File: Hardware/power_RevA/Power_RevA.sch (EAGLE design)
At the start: 11 parts, among them Q401 TIP120

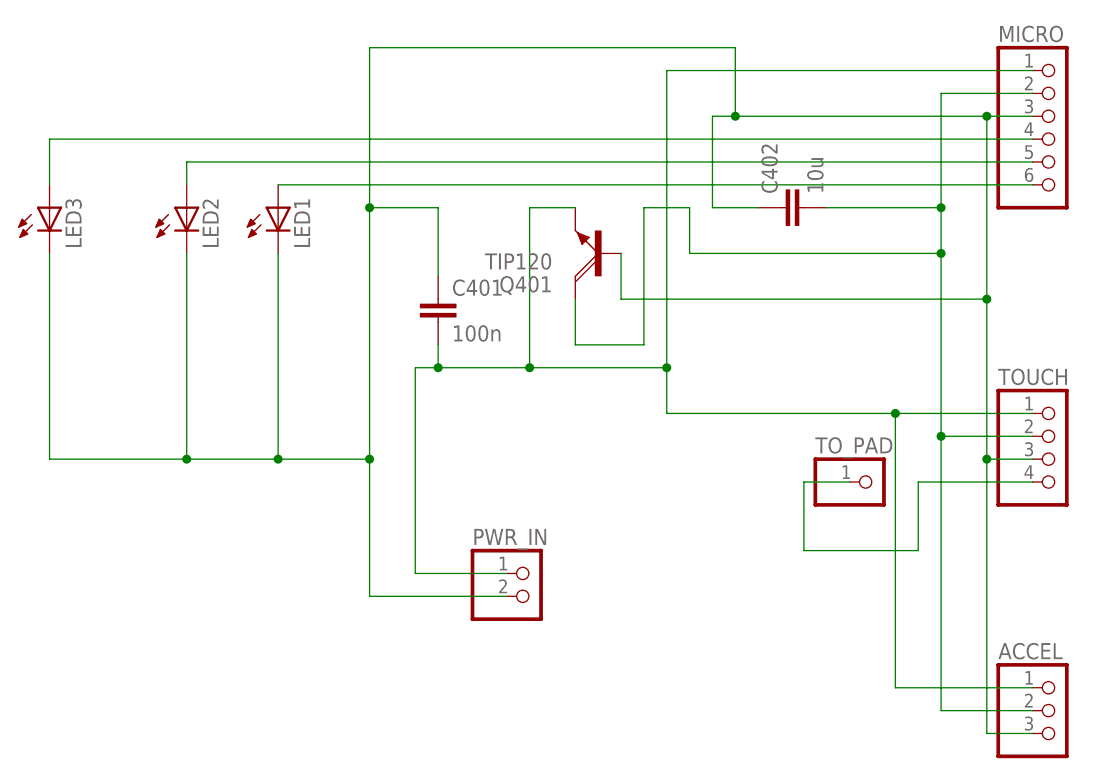
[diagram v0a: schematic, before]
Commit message: Power and Touch Board LED Orientation Fixed
The touch board is sill routed incorrectly (schematic is wrong too) but
orientation is silk-screened on board. Power board is routed absolutely
correctly.
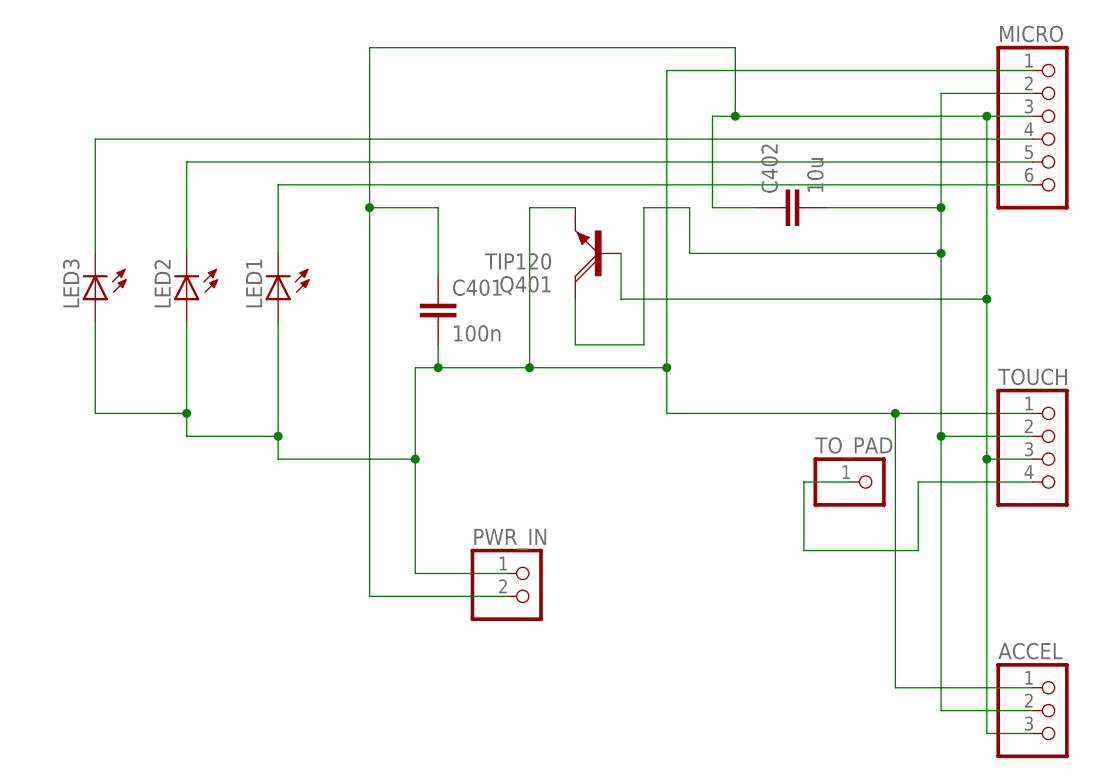
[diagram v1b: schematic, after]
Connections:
- removed net N$7: LED1.A, MICRO.6
- new net N$3: LED1.C, MICRO.6
- net N$2: now also LED1.A, LED2.A, LED3.A
- net N$5: now also LED2.C, MICRO.5; no longer LED3.A, MICRO.4
- net N$6: now also LED3.C, MICRO.4; no longer LED2.A, MICRO.5
- net N$8: no longer LED1.C, LED2.C, LED3.C
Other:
- moved on the sheet: LED1, LED2, LED3
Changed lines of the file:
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@@
 <instance part="TO_PAD" gate="G$1" x="86.36" y="33.02"/>
 <instance part="Q401" gate="1" x="55.88" y="58.42" rot="R180"/>
-<instance part="LED1" gate="G$1" x="20.32" y="63.5"/>
-<instance part="LED2" gate="G$1" x="10.16" y="63.5"/>
-<instance part="LED3" gate="G$1" x="-5.08" y="63.5"/>
+<instance part="LED1" gate="G$1" x="20.32" y="53.34" rot="R180"/>
+<instance part="LED2" gate="G$1" x="10.16" y="53.34" rot="R180"/>
+<instance part="LED3" gate="G$1" x="0" y="53.34" rot="R180"/>
 <instance part="C401" gate="G$1" x="38.1" y="53.34"/>
 <instance part="C402" gate="G$1" x="76.2" y="63.5" rot="R90"/>
@@
 <pinref part="PWR_IN" gate="G$1" pin="1"/>
 <wire x1="45.72" y1="22.86" x2="35.56" y2="22.86" width="0.1524" layer="91"/>
-<wire x1="35.56" y1="22.86" x2="35.56" y2="45.72" width="0.1524" layer="91"/>
+<wire x1="35.56" y1="22.86" x2="35.56" y2="35.56" width="0.1524" layer="91"/>
+<wire x1="35.56" y1="35.56" x2="35.56" y2="45.72" width="0.1524" layer="91"/>
 <wire x1="35.56" y1="45.72" x2="38.1" y2="45.72" width="0.1524" layer="91"/>
 <wire x1="38.1" y1="45.72" x2="48.26" y2="45.72" width="0.1524" layer="91"/>
@@
 <wire x1="48.26" y1="63.5" x2="48.26" y2="45.72" width="0.1524" layer="91"/>
 <junction x="48.26" y="45.72"/>
+<pinref part="LED1" gate="G$1" pin="A"/>
+<wire x1="20.32" y1="50.8" x2="20.32" y2="38.1" width="0.1524" layer="91"/>
+<wire x1="20.32" y1="38.1" x2="20.32" y2="35.56" width="0.1524" layer="91"/>
+<wire x1="20.32" y1="35.56" x2="35.56" y2="35.56" width="0.1524" layer="91"/>
+<junction x="35.56" y="35.56"/>
+<pinref part="LED2" gate="G$1" pin="A"/>
+<wire x1="10.16" y1="50.8" x2="10.16" y2="40.64" width="0.1524" layer="91"/>
+<wire x1="10.16" y1="40.64" x2="10.16" y2="38.1" width="0.1524" layer="91"/>
+<wire x1="10.16" y1="38.1" x2="20.32" y2="38.1" width="0.1524" layer="91"/>
+<junction x="20.32" y="38.1"/>
+<pinref part="LED3" gate="G$1" pin="A"/>
+<wire x1="0" y1="50.8" x2="0" y2="40.64" width="0.1524" layer="91"/>
+<wire x1="0" y1="40.64" x2="10.16" y2="40.64" width="0.1524" layer="91"/>
+<junction x="10.16" y="40.64"/>
 </segment>
 </net>
@@
 </segment>
 </net>
-<net name="N$5" class="0">
-<segment>
-<pinref part="MICRO" gate="A" pin="4"/>
-<pinref part="LED3" gate="G$1" pin="A"/>
-<wire x1="104.14" y1="71.12" x2="-5.08" y2="71.12" width="0.1524" layer="91"/>
-<wire x1="-5.08" y1="71.12" x2="-5.08" y2="66.04" width="0.1524" layer="91"/>
-</segment>
-</net>
-<net name="N$6" class="0">
-<segment>
-<pinref part="MICRO" gate="A" pin="5"/>
-<pinref part="LED2" gate="G$1" pin="A"/>
-<wire x1="104.14" y1="68.58" x2="10.16" y2="68.58" width="0.1524" layer="91"/>
-<wire x1="10.16" y1="68.58" x2="10.16" y2="66.04" width="0.1524" layer="91"/>
-</segment>
-</net>
-<net name="N$7" class="0">
-<segment>
-<pinref part="MICRO" gate="A" pin="6"/>
-<pinref part="LED1" gate="G$1" pin="A"/>
-<wire x1="104.14" y1="66.04" x2="20.32" y2="66.04" width="0.1524" layer="91"/>
-</segment>
-</net>
 <net name="N$8" class="0">
 <segment>
@@
 <junction x="71.12" y="73.66"/>
 <wire x1="38.1" y1="63.5" x2="30.48" y2="63.5" width="0.1524" layer="91"/>
-<wire x1="30.48" y1="63.5" x2="30.48" y2="35.56" width="0.1524" layer="91"/>
+<wire x1="30.48" y1="63.5" x2="30.48" y2="20.32" width="0.1524" layer="91"/>
 <pinref part="PWR_IN" gate="G$1" pin="2"/>
-<wire x1="30.48" y1="35.56" x2="30.48" y2="20.32" width="0.1524" layer="91"/>
 <wire x1="30.48" y1="20.32" x2="45.72" y2="20.32" width="0.1524" layer="91"/>
-<pinref part="LED1" gate="G$1" pin="C"/>
-<wire x1="20.32" y1="58.42" x2="20.32" y2="35.56" width="0.1524" layer="91"/>
-<wire x1="20.32" y1="35.56" x2="30.48" y2="35.56" width="0.1524" layer="91"/>
-<junction x="30.48" y="35.56"/>
-<pinref part="LED2" gate="G$1" pin="C"/>
-<wire x1="10.16" y1="58.42" x2="10.16" y2="35.56" width="0.1524" layer="91"/>
-<wire x1="10.16" y1="35.56" x2="20.32" y2="35.56" width="0.1524" layer="91"/>
-<junction x="20.32" y="35.56"/>
-<pinref part="LED3" gate="G$1" pin="C"/>
-<wire x1="-5.08" y1="58.42" x2="-5.08" y2="35.56" width="0.1524" layer="91"/>
-<wire x1="-5.08" y1="35.56" x2="10.16" y2="35.56" width="0.1524" layer="91"/>
-<junction x="10.16" y="35.56"/>
 <pinref part="C401" gate="G$1" pin="1"/>
 <wire x1="38.1" y1="55.88" x2="38.1" y2="63.5" width="0.1524" layer="91"/>
@@
 </segment>
 </net>
+<net name="N$3" class="0">
+<segment>
+<pinref part="LED1" gate="G$1" pin="C"/>
+<pinref part="MICRO" gate="A" pin="6"/>
+<wire x1="20.32" y1="58.42" x2="20.32" y2="66.04" width="0.1524" layer="91"/>
+<wire x1="20.32" y1="66.04" x2="104.14" y2="66.04" width="0.1524" layer="91"/>
+</segment>
+</net>
+<net name="N$5" class="0">
+<segment>
+<pinref part="LED2" gate="G$1" pin="C"/>
+<pinref part="MICRO" gate="A" pin="5"/>
+<wire x1="10.16" y1="58.42" x2="10.16" y2="68.58" width="0.1524" layer="91"/>
+<wire x1="10.16" y1="68.58" x2="104.14" y2="68.58" width="0.1524" layer="91"/>
+</segment>
+</net>
+<net name="N$6" class="0">
+<segment>
+<pinref part="LED3" gate="G$1" pin="C"/>
+<pinref part="MICRO" gate="A" pin="4"/>
+<wire x1="0" y1="58.42" x2="0" y2="71.12" width="0.1524" layer="91"/>
+<wire x1="0" y1="71.12" x2="104.14" y2="71.12" width="0.1524" layer="91"/>
+</segment>
+</net>

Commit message: Added Javen's logo to everything
Still need to add plus/minus on leds before order.
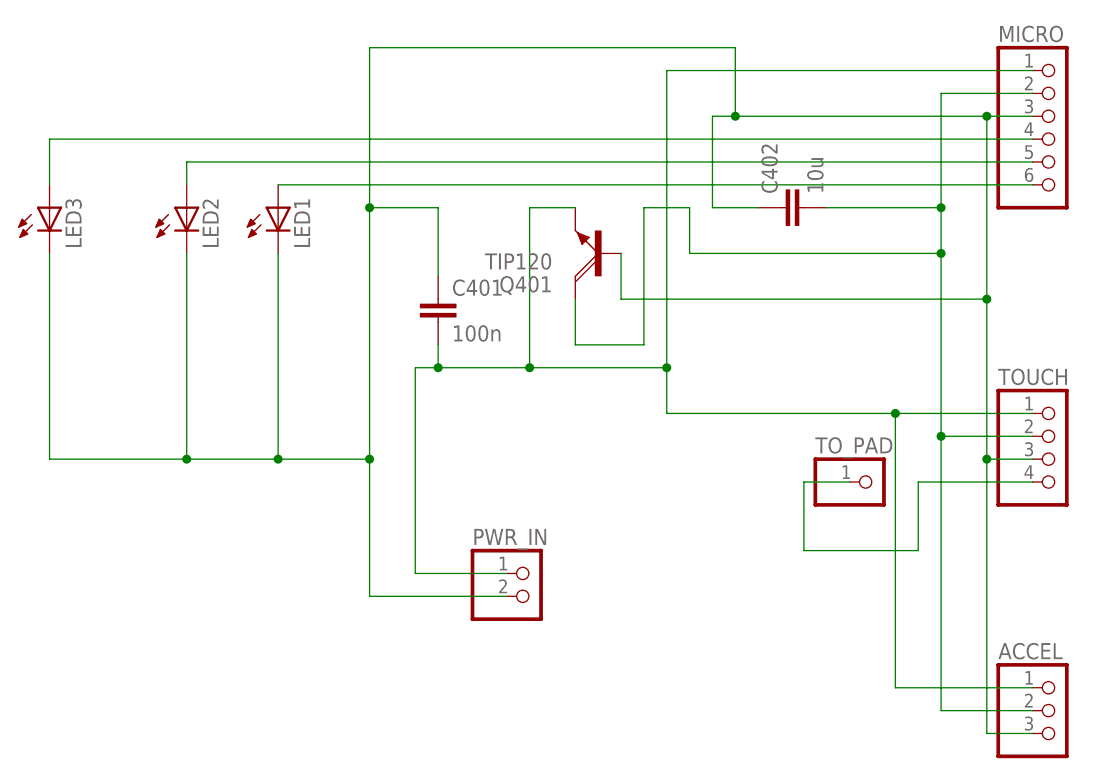
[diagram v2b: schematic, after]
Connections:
- removed net N$3: LED1.C, MICRO.6
- new net N$7: LED1.A, MICRO.6
- net N$2: no longer LED1.A, LED2.A, LED3.A
- net N$5: now also LED3.A, MICRO.4; no longer LED2.C, MICRO.5
- net N$6: now also LED2.A, MICRO.5; no longer LED3.C, MICRO.4
- net N$8: now also LED1.C, LED2.C, LED3.C
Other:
- moved on the sheet: LED1, LED2, LED3
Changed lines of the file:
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@@
 <instance part="TO_PAD" gate="G$1" x="86.36" y="33.02"/>
 <instance part="Q401" gate="1" x="55.88" y="58.42" rot="R180"/>
-<instance part="LED1" gate="G$1" x="20.32" y="53.34" rot="R180"/>
-<instance part="LED2" gate="G$1" x="10.16" y="53.34" rot="R180"/>
-<instance part="LED3" gate="G$1" x="0" y="53.34" rot="R180"/>
+<instance part="LED1" gate="G$1" x="20.32" y="63.5"/>
+<instance part="LED2" gate="G$1" x="10.16" y="63.5"/>
+<instance part="LED3" gate="G$1" x="-5.08" y="63.5"/>
 <instance part="C401" gate="G$1" x="38.1" y="53.34"/>
 <instance part="C402" gate="G$1" x="76.2" y="63.5" rot="R90"/>
@@
 <pinref part="PWR_IN" gate="G$1" pin="1"/>
 <wire x1="45.72" y1="22.86" x2="35.56" y2="22.86" width="0.1524" layer="91"/>
-<wire x1="35.56" y1="22.86" x2="35.56" y2="35.56" width="0.1524" layer="91"/>
-<wire x1="35.56" y1="35.56" x2="35.56" y2="45.72" width="0.1524" layer="91"/>
+<wire x1="35.56" y1="22.86" x2="35.56" y2="45.72" width="0.1524" layer="91"/>
 <wire x1="35.56" y1="45.72" x2="38.1" y2="45.72" width="0.1524" layer="91"/>
 <wire x1="38.1" y1="45.72" x2="48.26" y2="45.72" width="0.1524" layer="91"/>
@@
 <wire x1="48.26" y1="63.5" x2="48.26" y2="45.72" width="0.1524" layer="91"/>
 <junction x="48.26" y="45.72"/>
-<pinref part="LED1" gate="G$1" pin="A"/>
-<wire x1="20.32" y1="50.8" x2="20.32" y2="38.1" width="0.1524" layer="91"/>
-<wire x1="20.32" y1="38.1" x2="20.32" y2="35.56" width="0.1524" layer="91"/>
-<wire x1="20.32" y1="35.56" x2="35.56" y2="35.56" width="0.1524" layer="91"/>
-<junction x="35.56" y="35.56"/>
-<pinref part="LED2" gate="G$1" pin="A"/>
-<wire x1="10.16" y1="50.8" x2="10.16" y2="40.64" width="0.1524" layer="91"/>
-<wire x1="10.16" y1="40.64" x2="10.16" y2="38.1" width="0.1524" layer="91"/>
-<wire x1="10.16" y1="38.1" x2="20.32" y2="38.1" width="0.1524" layer="91"/>
-<junction x="20.32" y="38.1"/>
-<pinref part="LED3" gate="G$1" pin="A"/>
-<wire x1="0" y1="50.8" x2="0" y2="40.64" width="0.1524" layer="91"/>
-<wire x1="0" y1="40.64" x2="10.16" y2="40.64" width="0.1524" layer="91"/>
-<junction x="10.16" y="40.64"/>
 </segment>
 </net>
@@
 </segment>
 </net>
+<net name="N$5" class="0">
+<segment>
+<pinref part="MICRO" gate="A" pin="4"/>
+<pinref part="LED3" gate="G$1" pin="A"/>
+<wire x1="104.14" y1="71.12" x2="-5.08" y2="71.12" width="0.1524" layer="91"/>
+<wire x1="-5.08" y1="71.12" x2="-5.08" y2="66.04" width="0.1524" layer="91"/>
+</segment>
+</net>
+<net name="N$6" class="0">
+<segment>
+<pinref part="MICRO" gate="A" pin="5"/>
+<pinref part="LED2" gate="G$1" pin="A"/>
+<wire x1="104.14" y1="68.58" x2="10.16" y2="68.58" width="0.1524" layer="91"/>
+<wire x1="10.16" y1="68.58" x2="10.16" y2="66.04" width="0.1524" layer="91"/>
+</segment>
+</net>
+<net name="N$7" class="0">
+<segment>
+<pinref part="MICRO" gate="A" pin="6"/>
+<pinref part="LED1" gate="G$1" pin="A"/>
+<wire x1="104.14" y1="66.04" x2="20.32" y2="66.04" width="0.1524" layer="91"/>
+</segment>
+</net>
 <net name="N$8" class="0">
 <segment>
@@
 <junction x="71.12" y="73.66"/>
 <wire x1="38.1" y1="63.5" x2="30.48" y2="63.5" width="0.1524" layer="91"/>
-<wire x1="30.48" y1="63.5" x2="30.48" y2="20.32" width="0.1524" layer="91"/>
+<wire x1="30.48" y1="63.5" x2="30.48" y2="35.56" width="0.1524" layer="91"/>
 <pinref part="PWR_IN" gate="G$1" pin="2"/>
+<wire x1="30.48" y1="35.56" x2="30.48" y2="20.32" width="0.1524" layer="91"/>
 <wire x1="30.48" y1="20.32" x2="45.72" y2="20.32" width="0.1524" layer="91"/>
+<pinref part="LED1" gate="G$1" pin="C"/>
+<wire x1="20.32" y1="58.42" x2="20.32" y2="35.56" width="0.1524" layer="91"/>
+<wire x1="20.32" y1="35.56" x2="30.48" y2="35.56" width="0.1524" layer="91"/>
+<junction x="30.48" y="35.56"/>
+<pinref part="LED2" gate="G$1" pin="C"/>
+<wire x1="10.16" y1="58.42" x2="10.16" y2="35.56" width="0.1524" layer="91"/>
+<wire x1="10.16" y1="35.56" x2="20.32" y2="35.56" width="0.1524" layer="91"/>
+<junction x="20.32" y="35.56"/>
+<pinref part="LED3" gate="G$1" pin="C"/>
+<wire x1="-5.08" y1="58.42" x2="-5.08" y2="35.56" width="0.1524" layer="91"/>
+<wire x1="-5.08" y1="35.56" x2="10.16" y2="35.56" width="0.1524" layer="91"/>
+<junction x="10.16" y="35.56"/>
 <pinref part="C401" gate="G$1" pin="1"/>
 <wire x1="38.1" y1="55.88" x2="38.1" y2="63.5" width="0.1524" layer="91"/>
@@
 </segment>
 </net>
-<net name="N$3" class="0">
-<segment>
-<pinref part="LED1" gate="G$1" pin="C"/>
-<pinref part="MICRO" gate="A" pin="6"/>
-<wire x1="20.32" y1="58.42" x2="20.32" y2="66.04" width="0.1524" layer="91"/>
-<wire x1="20.32" y1="66.04" x2="104.14" y2="66.04" width="0.1524" layer="91"/>
-</segment>
-</net>
-<net name="N$5" class="0">
-<segment>
-<pinref part="LED2" gate="G$1" pin="C"/>
-<pinref part="MICRO" gate="A" pin="5"/>
-<wire x1="10.16" y1="58.42" x2="10.16" y2="68.58" width="0.1524" layer="91"/>
-<wire x1="10.16" y1="68.58" x2="104.14" y2="68.58" width="0.1524" layer="91"/>
-</segment>
-</net>
-<net name="N$6" class="0">
-<segment>
-<pinref part="LED3" gate="G$1" pin="C"/>
-<pinref part="MICRO" gate="A" pin="4"/>
-<wire x1="0" y1="58.42" x2="0" y2="71.12" width="0.1524" layer="91"/>
-<wire x1="0" y1="71.12" x2="104.14" y2="71.12" width="0.1524" layer="91"/>
-</segment>
-</net>
